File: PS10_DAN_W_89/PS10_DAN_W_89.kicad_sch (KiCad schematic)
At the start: 13 parts, among them J1 Conn_01x15_Pin, J2 IDC26, Q1 BUZ11F1 x 2pcs., Q2 BUZ11F1 x 2pcs., Q3 BUZ11F1 x 2pcs., Q4 BUZ11F1 x 2pcs.

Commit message: Documentation cont.
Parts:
- removed RN1: R_Network09_US, Resistor_THT:R_Array_SIP10, symbol Device:R_Network09_US
- added U1: AD7545, symbol kpole:AD7545
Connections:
- net at J2.10 (Pin_10): now also U1.10 (DB5)
- net at J2.11 (Pin_11): now also U1.12 (DB3)
- net at J2.12 (Pin_12): now also U1.9 (DB6)
- net at J2.13 (Pin_13): now also U1.13 (DB2)
- net at J2.14 (Pin_14): now also U1.8 (DB7)
- net at J2.15 (Pin_15): now also U1.14 (DB1)
- net at J2.16 (Pin_16): now also U1.7 (DB8)
- net at J2.17 (Pin_17): now also U1.15 (DB0)
- net at J2.18 (Pin_18): now also U1.6 (DB9)
- net at J2.19 (Pin_19): now also U1.4 (DB11)
- net at J2.20 (Pin_20): now also U1.5 (DB10)
- net at J2.9 (Pin_9): now also U1.11 (DB4)
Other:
- moved on the sheet: C1, C2, C3, C4, C5, J1, J2, L1, Q1, Q2, Q3, Q4

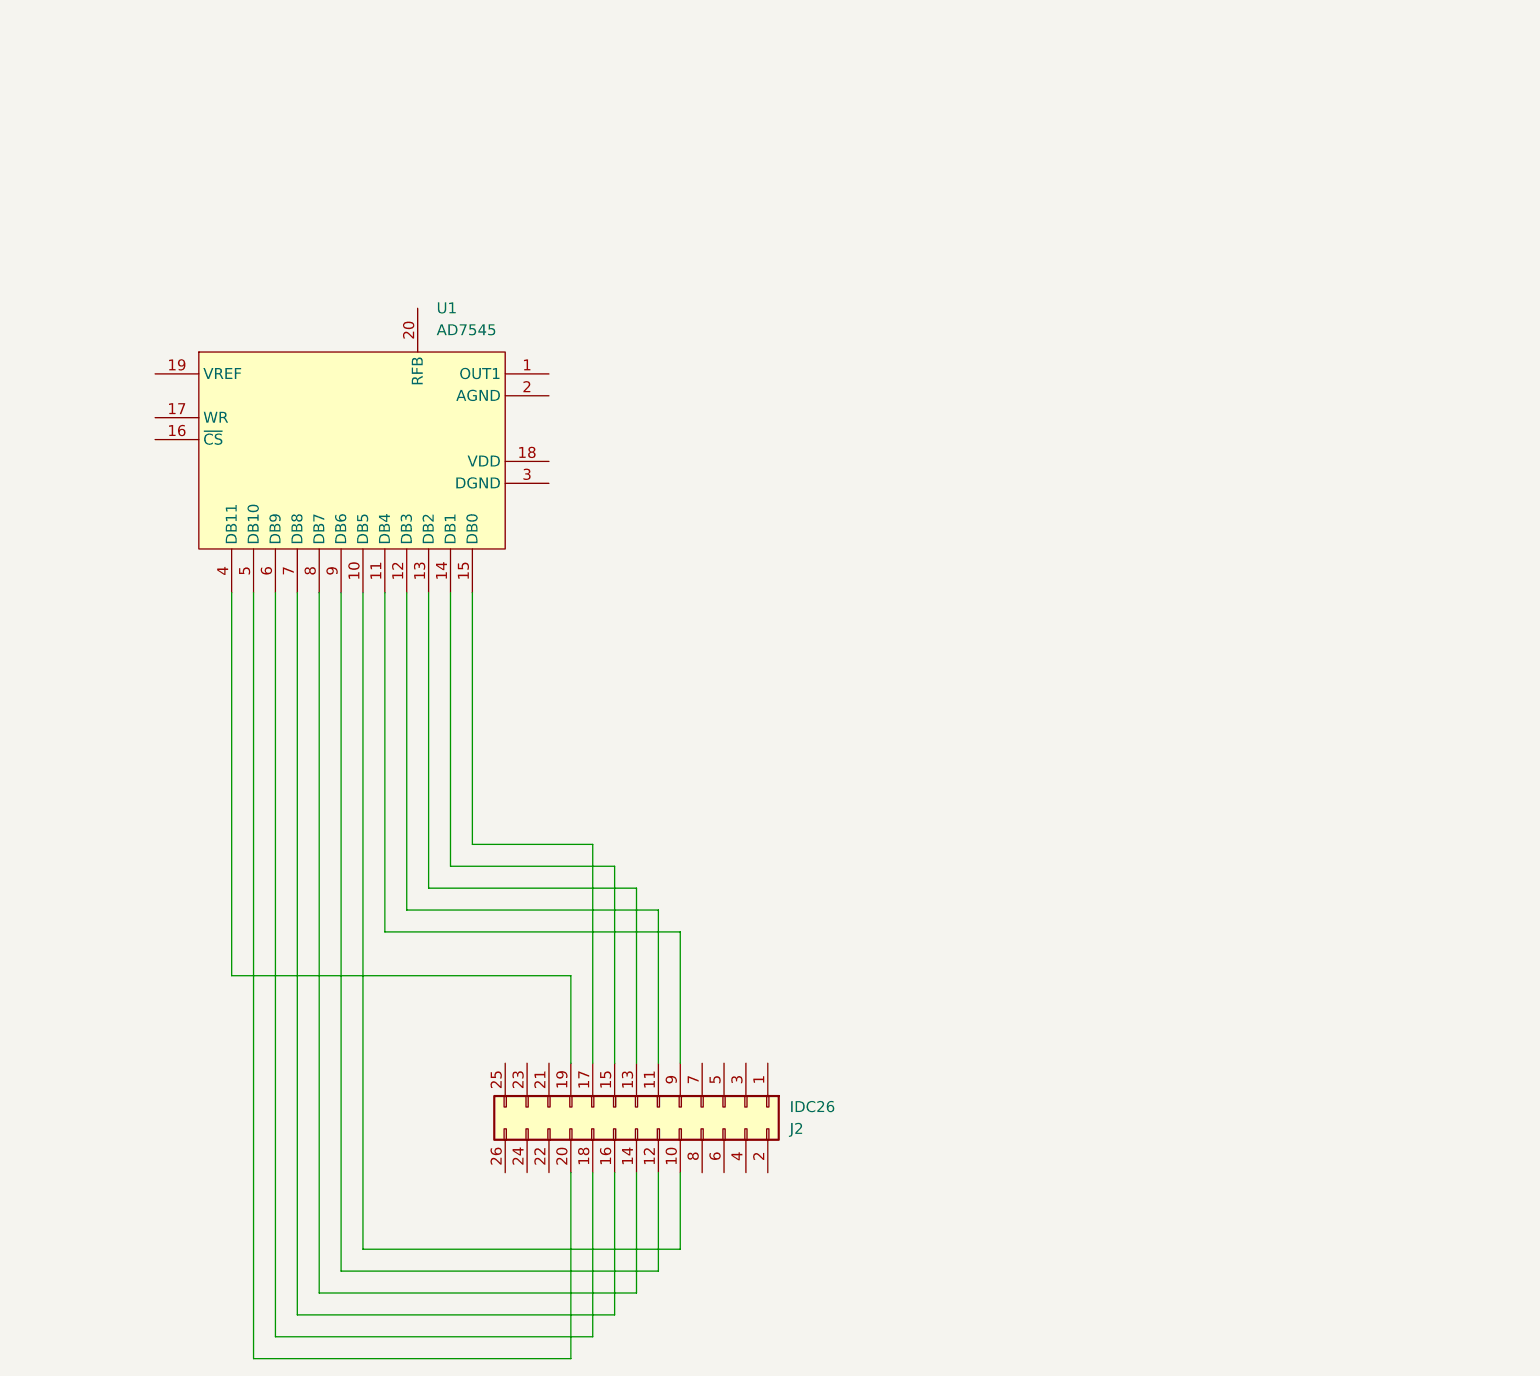
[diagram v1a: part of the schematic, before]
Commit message: Documentation cont.
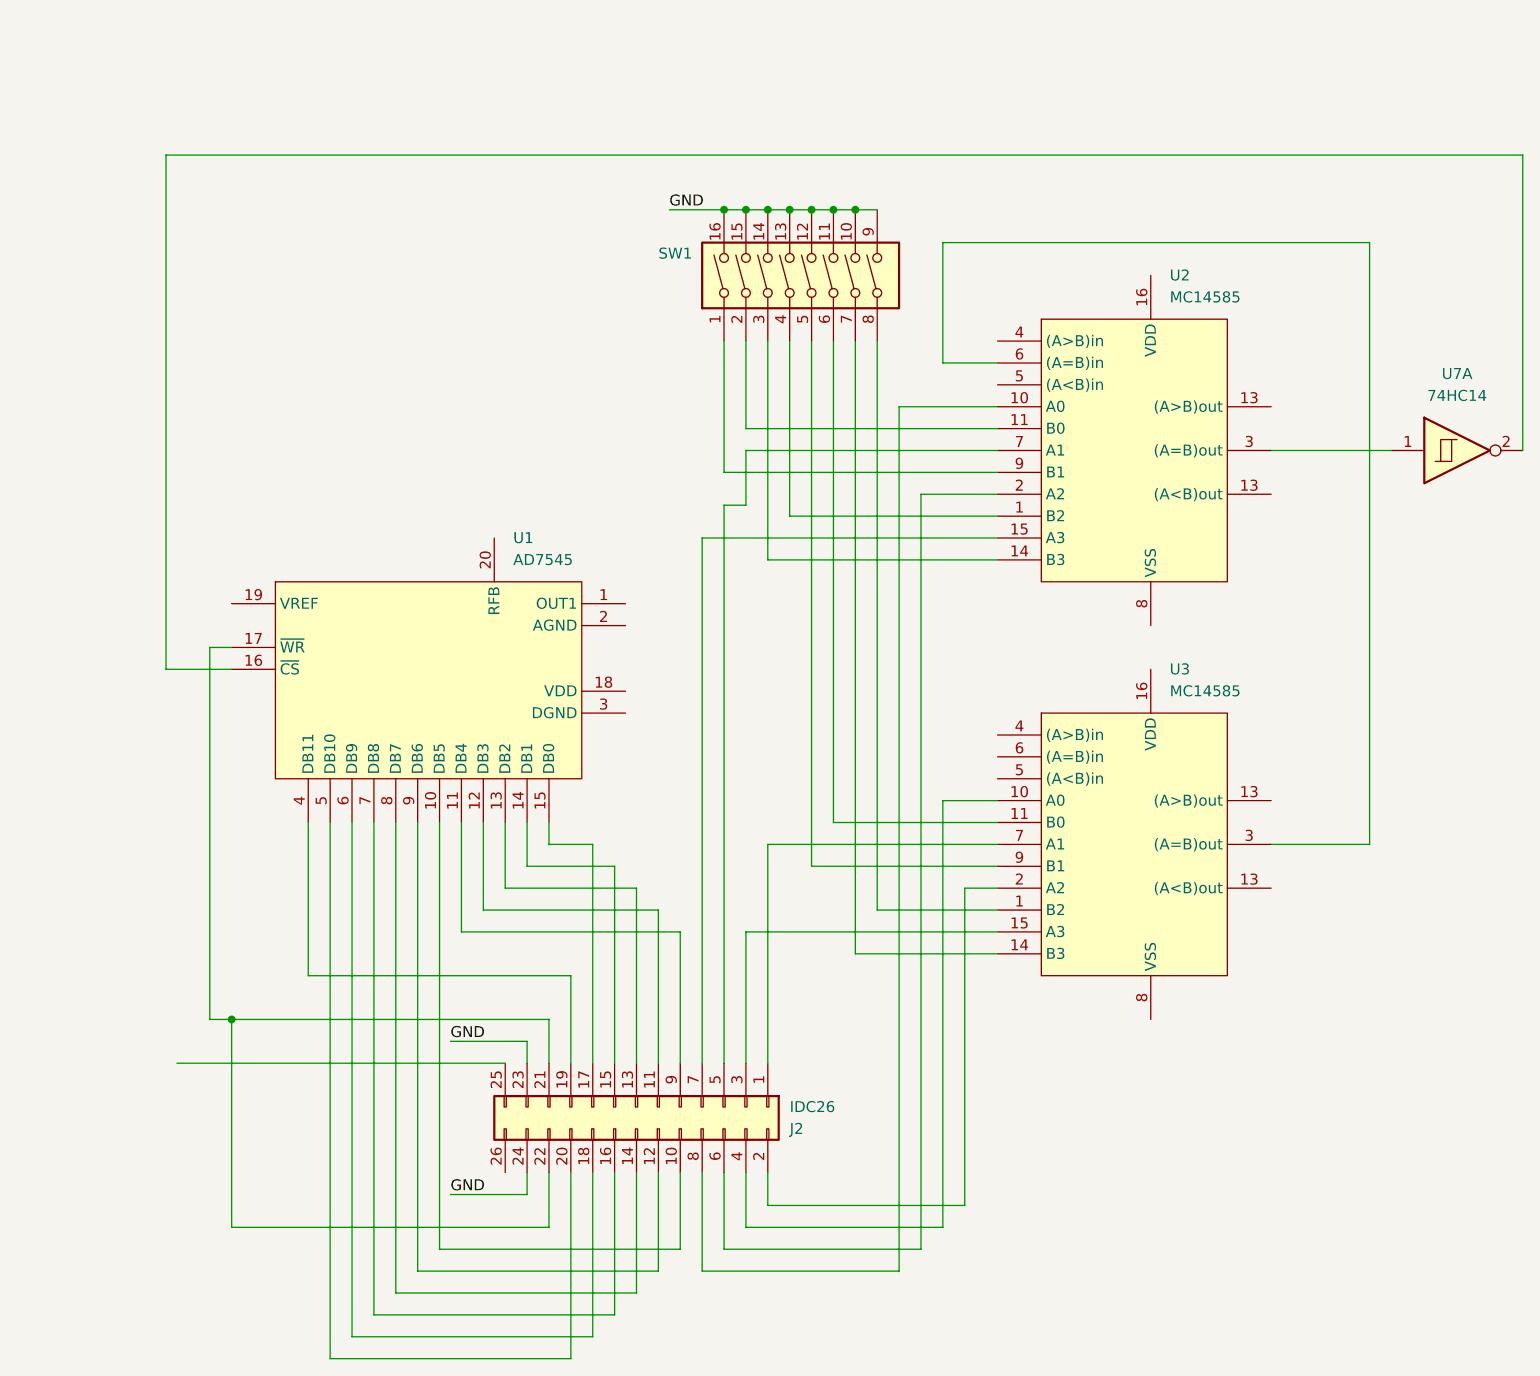
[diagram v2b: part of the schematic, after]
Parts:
- added SW1: SW_DIP_x08, symbol Switch:SW_DIP_x08
- added U2, U3: MC14585, symbol kpole:MC14585
- added U7: 74HC14, symbol 74xx:74HC14
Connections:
- net GND: now also J2.23 (Pin_23), J2.24 (Pin_24), SW1.10, SW1.11, SW1.12, SW1.13, SW1.14, SW1.15, SW1.16, SW1.9
- net at U1.16 (~{CS}): now also U7.2
- net at U1.17 (~{WR}): now also J2.21 (Pin_21), J2.22 (Pin_22)
- net at J2.1 (Pin_1): now also U3.7 (A1)
- net at J2.2 (Pin_2): now also U3.2 (A2)
- net at J2.3 (Pin_3): now also U3.15 (A3)
- net at J2.4 (Pin_4): now also U3.10 (A0)
- net at J2.5 (Pin_5): now also U2.7 (A1)
- net at J2.6 (Pin_6): now also U2.2 (A2)
- net at J2.7 (Pin_7): now also U2.15 (A3)
- net at J2.8 (Pin_8): now also U2.10 (A0)
- new net: SW1.4, U2.1 (B2)
- new net: SW1.2, U2.11 (B0)
- new net: SW1.3, U2.14 (B3)
- new net: U2.3 ((A=B)out), U7.1
- new net: U2.6 ((A=B)in), U3.3 ((A=B)out)
- new net: SW1.1, U2.9 (B1)
- new net: SW1.5, U3.9 (B1)
- new net: SW1.6, U3.11 (B0)
- new net: SW1.7, U3.14 (B3)
- new net: SW1.8, U3.1 (B2)
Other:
- moved on the sheet: U1
